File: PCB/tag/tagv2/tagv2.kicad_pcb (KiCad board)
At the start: 2 copper layers, 24.4 x 19.3 mm, 25 parts, among them J1 SM02B-SRSS-TB LFSN, J3 Conn_ARM_JTAG_SWD_10, J4 PRT-12807, Q1 IRLML2402TRPBF, Q2 IRLML2402TRPBF, U1 DWM3001C, U2 TPS79933DDCR

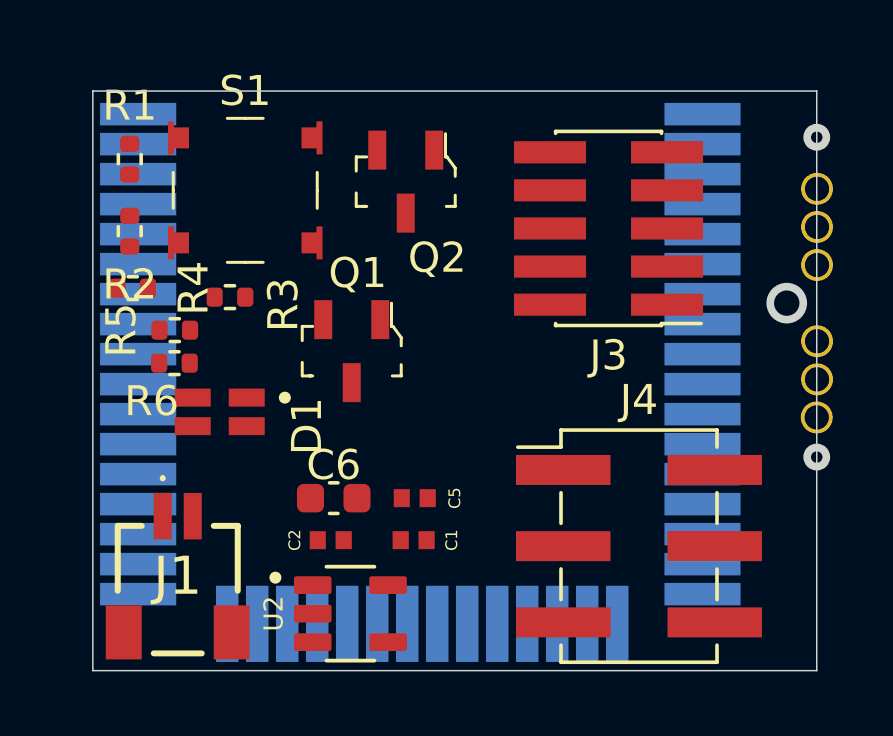
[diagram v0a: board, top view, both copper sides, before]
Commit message: new pcb
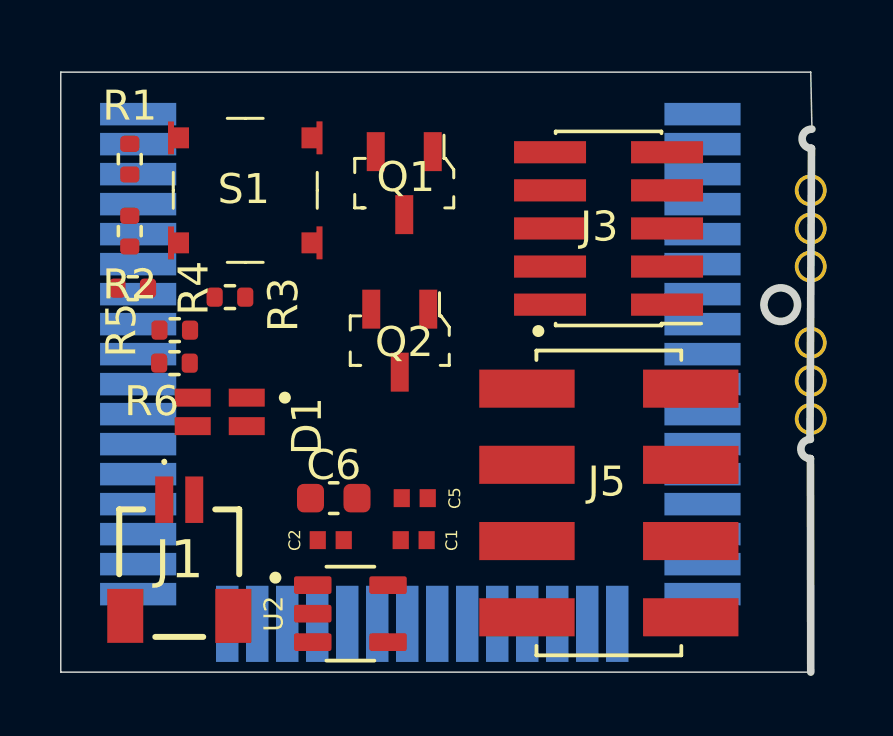
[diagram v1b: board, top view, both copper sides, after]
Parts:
- removed the ? at (76.2, 30.4)
- removed the ? at (76.2, 35.5)
- removed the ? at (76.2, 27.9)
- removed the ? at (76.2, 33.0)
- removed the ? at (76.2, 29.2)
- removed the ? at (76.2, 34.2)
- removed J4: PRT-12807, Connector_PinHeader_2.54mm:PinHeader_2x03_P2.54mm_Vertical_SMD
- added ?: , , F.Cu at (76.0, 29.2)
- added ?: , , F.Cu at (76.0, 35.6)
- added ?: , , F.Cu at (76.0, 30.5)
- added ?: , , F.Cu at (76.0, 33.0)
- added ?: , , F.Cu at (76.0, 27.9)
- added ?: , , F.Cu at (76.0, 34.3)
- added J5: 54202-T0804LF, imported:AMPHENOL_54202-T0804LF, F.Cu at (69.3, 38.4)
- moved Q1 5.87 mm to (62.5, 27.7)
- moved Q2 5.30 mm to (62.3, 33.0)
- moved J1 0.55 mm to (55.0, 40.5)
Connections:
- D1 pad 1: Net-(D1-K2) -> Net-(D1-A2)
- D1 pad 2: Net-(D1-A2) -> Net-(D1-K2)
- D1 pad 3: Net-(D1-A1) -> Net-(D1-K1)
- D1 pad 4: Net-(D1-K1) -> Net-(D1-A1)
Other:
- board size 24.4 x 19.3 mm -> 25 x 20 mm
